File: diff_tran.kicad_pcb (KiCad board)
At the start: 2 copper layers, 28.7 x 13.8 mm, 29 parts, among them IC1 SN65LVDM176, IC2 SN65LVDM176, IC3 SN65LVDM176, IC4 SN65LVDM176, J1 SOLDER_JUMPER, J10 SOLDER_JUMPER, J11 SOLDER_JUMPER, J12 SOLDER_JUMPER, J2 SOLDER_JUMPER, J3 SOLDER_JUMPER, J4 SOLDER_JUMPER, J5 SOLDER_JUMPER, J6 SOLDER_JUMPER, J7 SOLDER_JUMPER, J8 SOLDER_JUMPER, J9 SOLDER_JUMPER, P1 CONN_02X03, P2 CONN_02X05

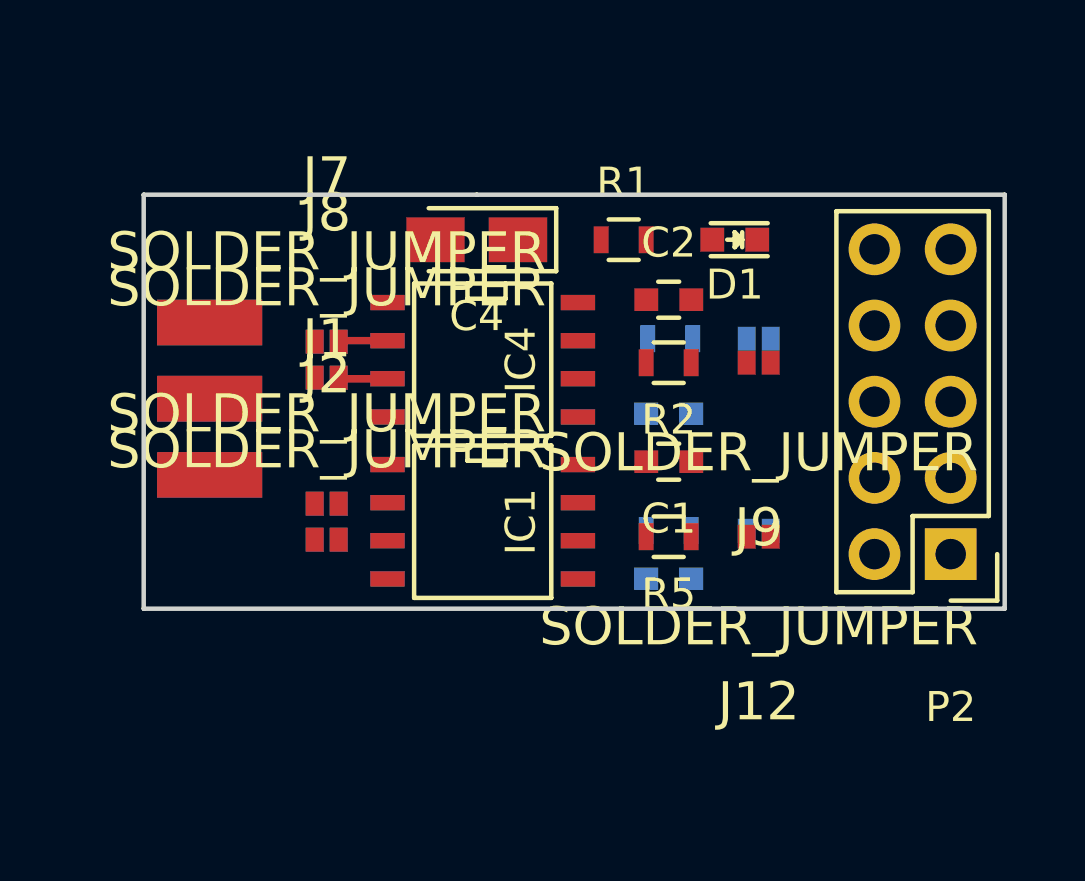
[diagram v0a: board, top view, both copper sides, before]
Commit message: Tracks
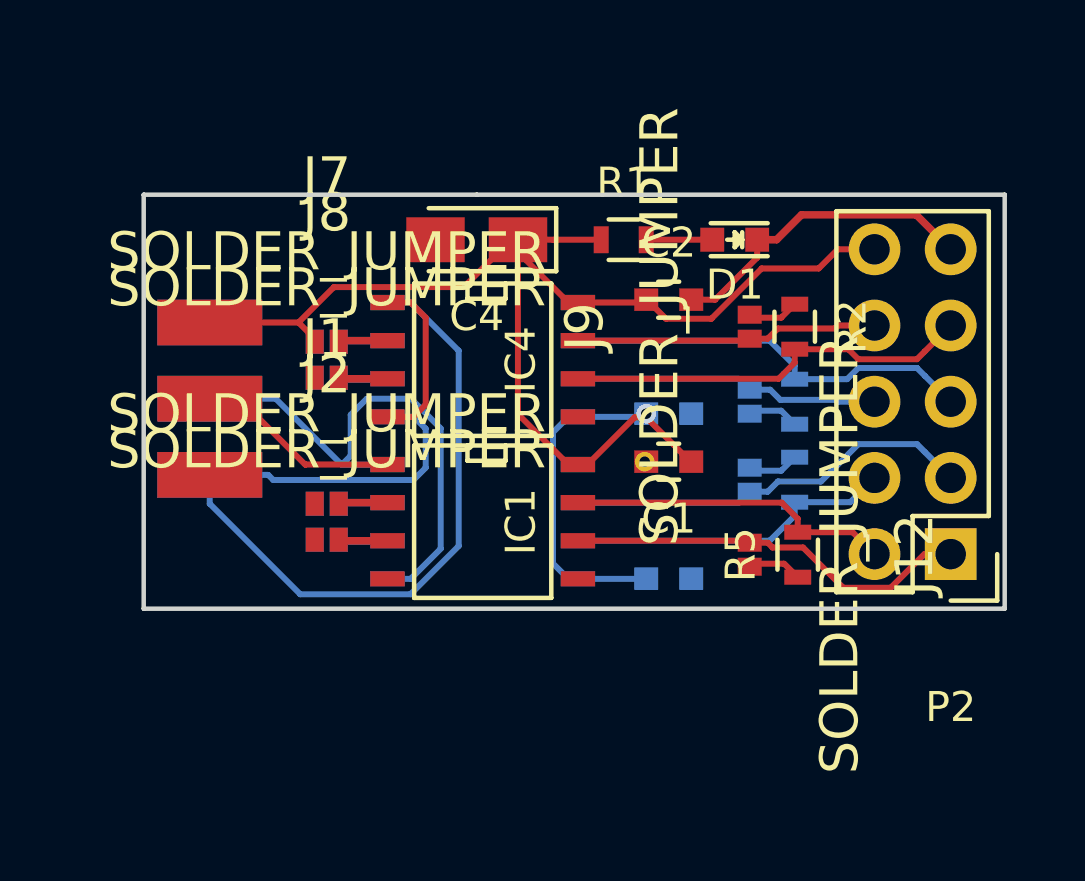
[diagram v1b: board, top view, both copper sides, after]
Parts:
- added ?: , LercheTech:Lerche_via_0.35_GND_MaskOver, F.Cu at (146.2, 98.9)
- moved R3 4.65 mm to (151.2, 96.9), turned to 90 degrees
- moved R4 4.53 mm to (151.2, 99.5), turned to 270 degrees
- moved R2 4.37 mm to (151.2, 94.4), turned to 270 degrees
- moved R5 4.34 mm to (151.3, 102.0), turned to 90 degrees
- moved J10 2.12 mm to (149.7, 96.9), turned to 270 degrees
- moved J11 1.73 mm to (149.7, 99.5), turned to 90 degrees
- moved J9 1.24 mm to (149.7, 94.4), turned to 90 degrees
- moved J12 0.67 mm to (149.7, 102.0), turned to 270 degrees
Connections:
- J12 pad 1: Net-(IC1-Pad7) -> Net-(IC1-Pad6)
- R5 pad 2: Net-(IC1-Pad6) -> Net-(IC1-Pad7)
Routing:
- net +3V3: track 0.00 -> 53.9 mm, vias 0 -> 1
- net MISO: track 0.00 -> 30.9 mm
- net MOSI: track 0.00 -> 18.5 mm
- net Net-(IC3-Pad6): track 0.00 -> 13.8 mm
- net Net-(IC4-Pad6): track 0.00 -> 13.7 mm
- net Net-(IC2-Pad6): track 0.00 -> 13.7 mm
- net Net-(IC1-Pad6): track 0.00 -> 13.5 mm
- net Net-(IC1-Pad7): track 0.00 -> 11.5 mm
- net Net-(IC2-Pad7): track 0.00 -> 11.0 mm
- net GND: track 0.00 -> 10.6 mm
- net Net-(IC3-Pad7): track 0.00 -> 10.2 mm
- net Net-(IC4-Pad7): track 0.00 -> 10.1 mm
- net SCK: track 0.00 -> 6.84 mm
- net SSEL: track 0.00 -> 5.83 mm
- net Net-(D1-Pad2): track 0.00 -> 2.20 mm
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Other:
- net class Default: clearance 0.2 -> 0.16; trace_width 0.25 -> 0.2
- rule trace_clearance: 0.2 -> 0.16
- rule trace_min: 0.2 -> 0.15
